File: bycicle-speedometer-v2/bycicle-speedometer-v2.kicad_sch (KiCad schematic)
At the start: 13 parts, among them J2 Conn_01x02_Pin, J3 Conn_01x02_Pin, SW1 SW_Push_Dual, U1 ESP-12E, U2 AMS1117-3.3

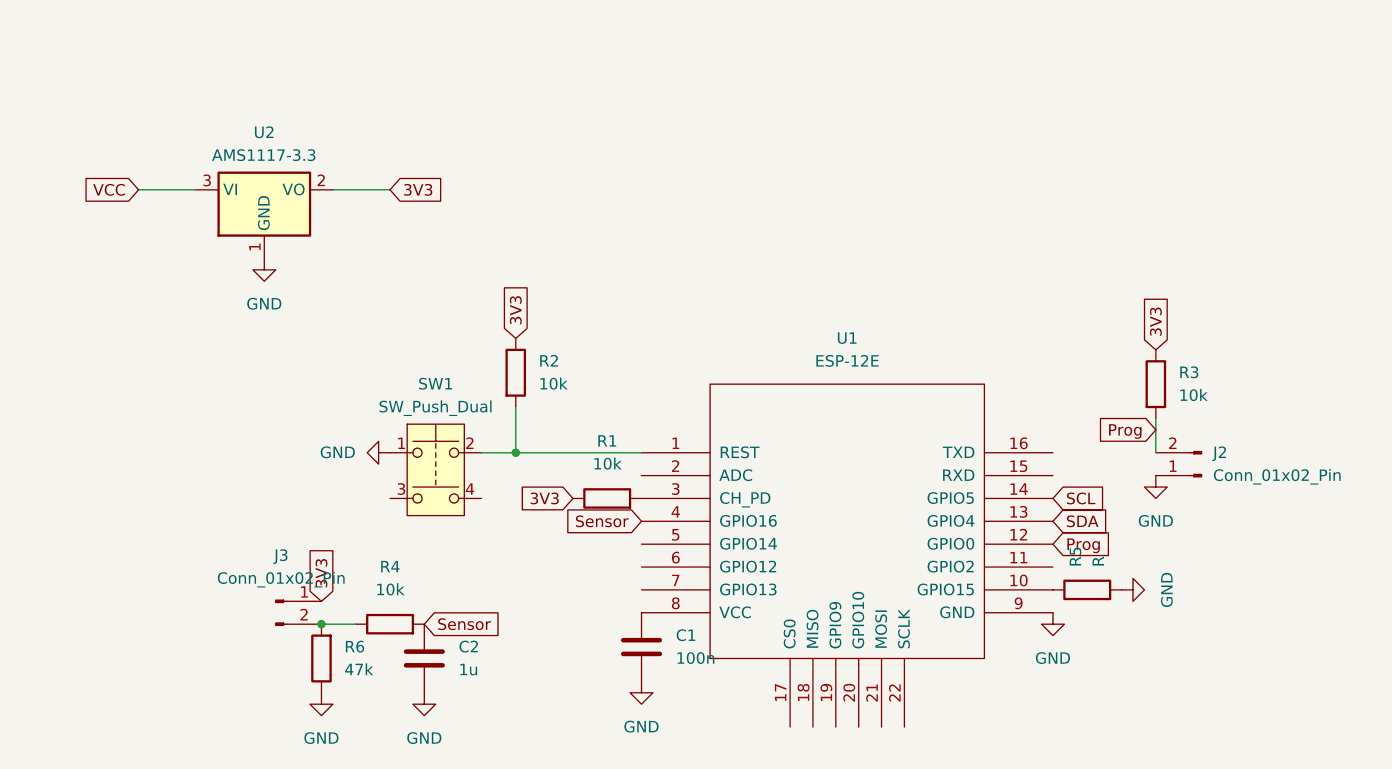
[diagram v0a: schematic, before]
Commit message: edited schematic diagram
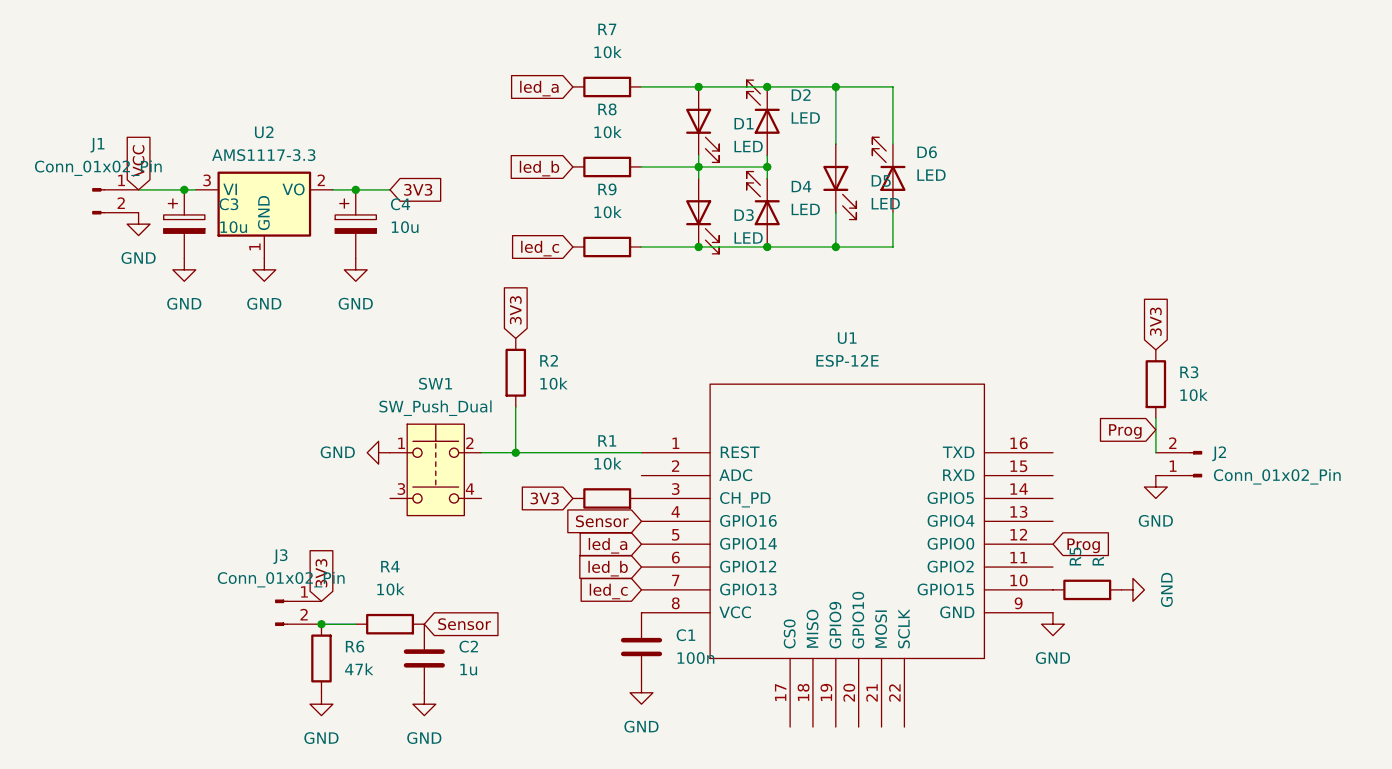
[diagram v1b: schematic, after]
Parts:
- added C3, C4: 10u, Capacitor_SMD:CP_Elec_5x4.5, symbol Device:C_Polarized
- added D1, D2, D3, D4, D5, D6: LED, LED_THT:LED_D5.0mm, symbol Device:LED
- added J1: Conn_01x02_Pin, TerminalBlock_Phoenix:TerminalBlock_Phoenix_MKDS-1,5-2-5.08_1x02_P5.08mm_Horizontal, symbol Connector:Conn_01x02_Pin
- added R7, R8, R9: 10k, Resistor_SMD:R_0805_2012Metric, symbol Device:R
- J3: footprint Connector_PinHeader_2.54mm:PinHeader_1x02_P2.54mm_Vertical -> TerminalBlock_Phoenix:TerminalBlock_Phoenix_MKDS-1,5-2-5.08_1x02_P5.08mm_Horizontal
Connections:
- net 3V3: now also C4.1
- net GND: now also C3.2, C4.2, J1.2 (Pin_2)
- net VCC: now also C3.1, J1.1 (Pin_1)
- net led_a: now reaches U1.5 (GPIO14)
- net led_a: now also R7.1
- net led_b: now reaches U1.6 (GPIO12)
- net led_b: now also R8.1
- net led_c: now reaches U1.7 (GPIO13)
- net led_c: now also R9.1
- net SCL: no longer names the net of U1.14 (GPIO5)
- net SDA: no longer names the net of U1.13 (GPIO4)
- new net: D1.2 (A), D2.1 (K), D5.2 (A), D6.1 (K), R7.2
- new net: D3.1 (K), D4.2 (A), D5.1 (K), D6.2 (A), R9.2
- new net: D1.1 (K), D2.2 (A), D3.2 (A), D4.1 (K), R8.2

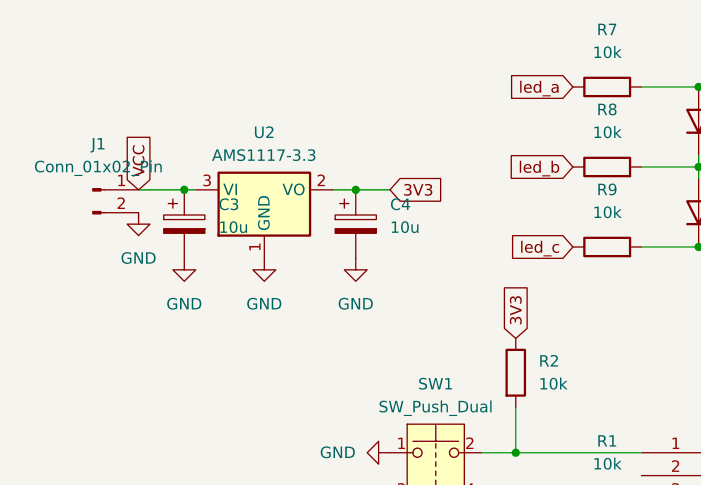
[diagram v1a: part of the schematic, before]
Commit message: edited schematics
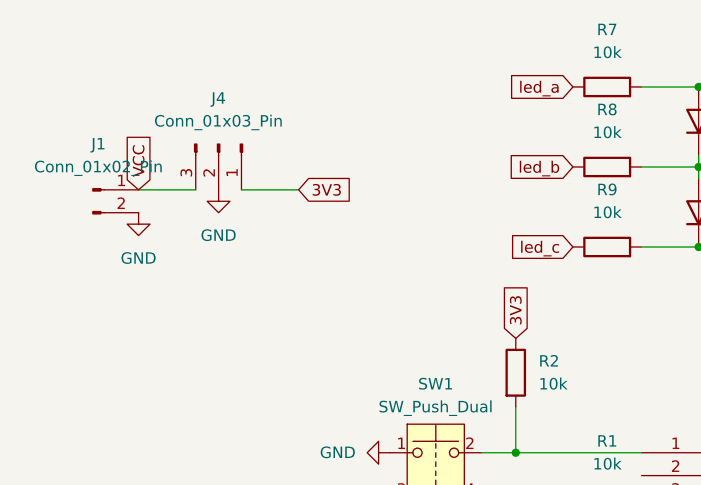
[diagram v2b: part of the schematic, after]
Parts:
- removed C3, C4: 10u, Capacitor_SMD:CP_Elec_5x4.5, symbol Device:C_Polarized
- removed U2: AMS1117-3.3, Package_TO_SOT_SMD:SOT-223-3_TabPin2, symbol Regulator_Linear:AMS1117-3.3
- added J4: Conn_01x03_Pin, Connector_PinHeader_2.54mm:PinHeader_1x03_P2.54mm_Vertical, symbol Connector:Conn_01x03_Pin
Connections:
- net 3V3: now also J4.1 (Pin_1)
- net GND: now also J4.2 (Pin_2)
- net VCC: now also J4.3 (Pin_3)
